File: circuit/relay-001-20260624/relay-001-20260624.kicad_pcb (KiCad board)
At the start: 2 copper layers, 169 x 126.3 mm, 15 parts, among them J1 Conn_01x03_Pin, J10 Conn_01x02_Pin, J11 Conn_01x02_Pin, J12 Conn_01x02_Pin, J13 Conn_01x02_Pin, J14 Conn_01x02_Pin, J15 Conn_01x02_Pin, J2 Conn_02x05_Odd_Even, J3 Conn_02x08_Odd_Even, J4 Conn_02x09_Odd_Even, J5 Conn_01x02_Pin, J6 Conn_01x02_Pin, J7 Conn_01x02_Pin, J8 Conn_01x02_Pin, J9 Conn_01x02_Pin

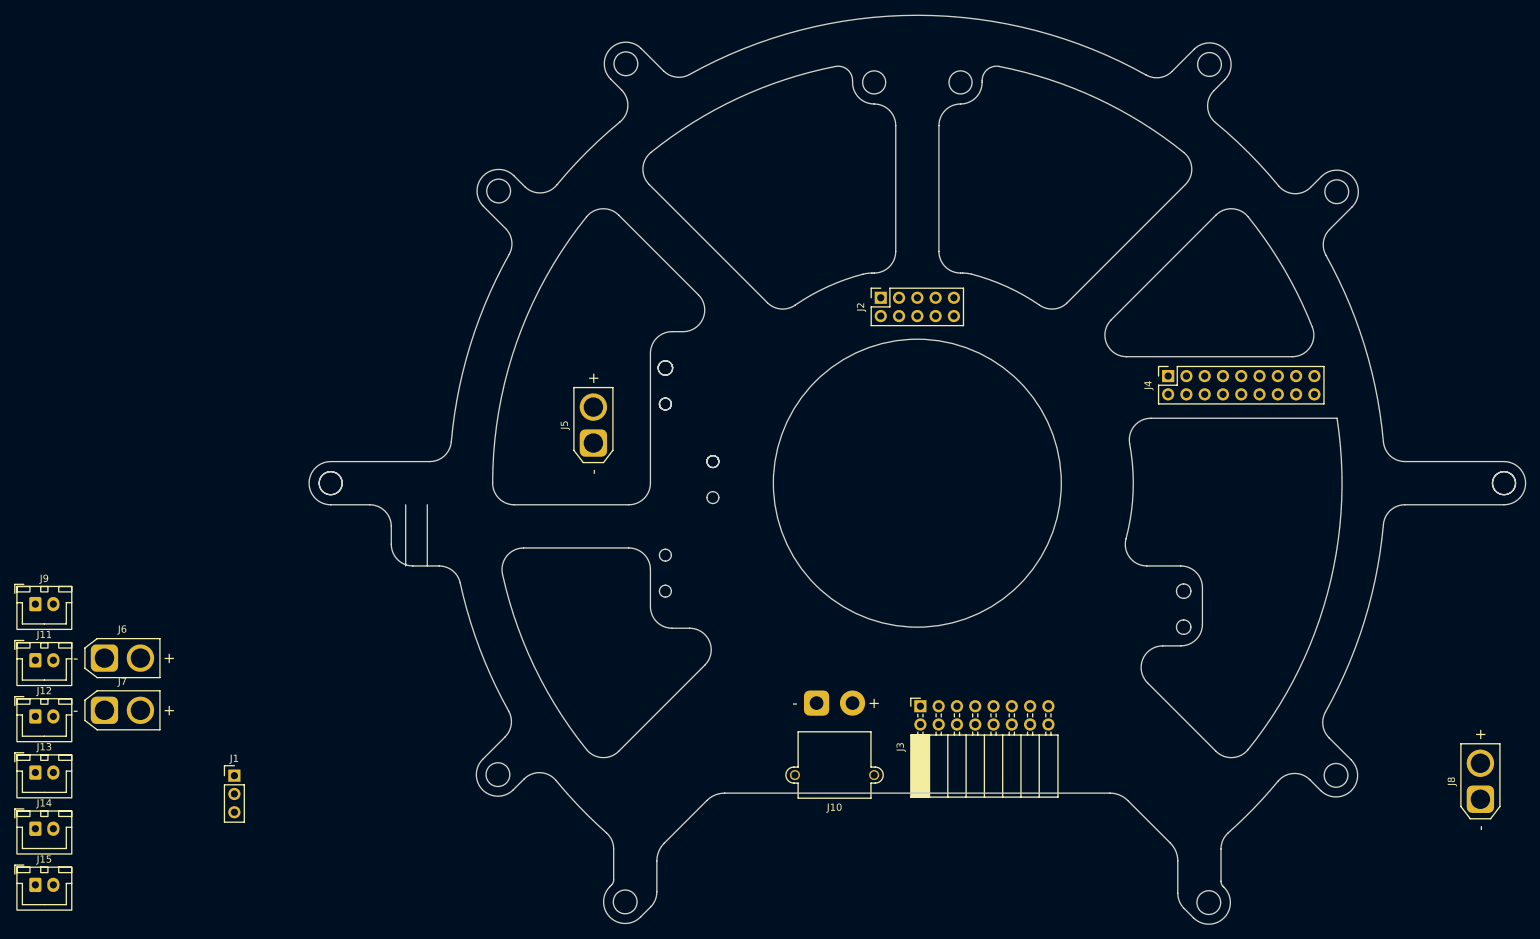
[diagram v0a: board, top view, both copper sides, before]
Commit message: Update 供給基板のボード図を進めた
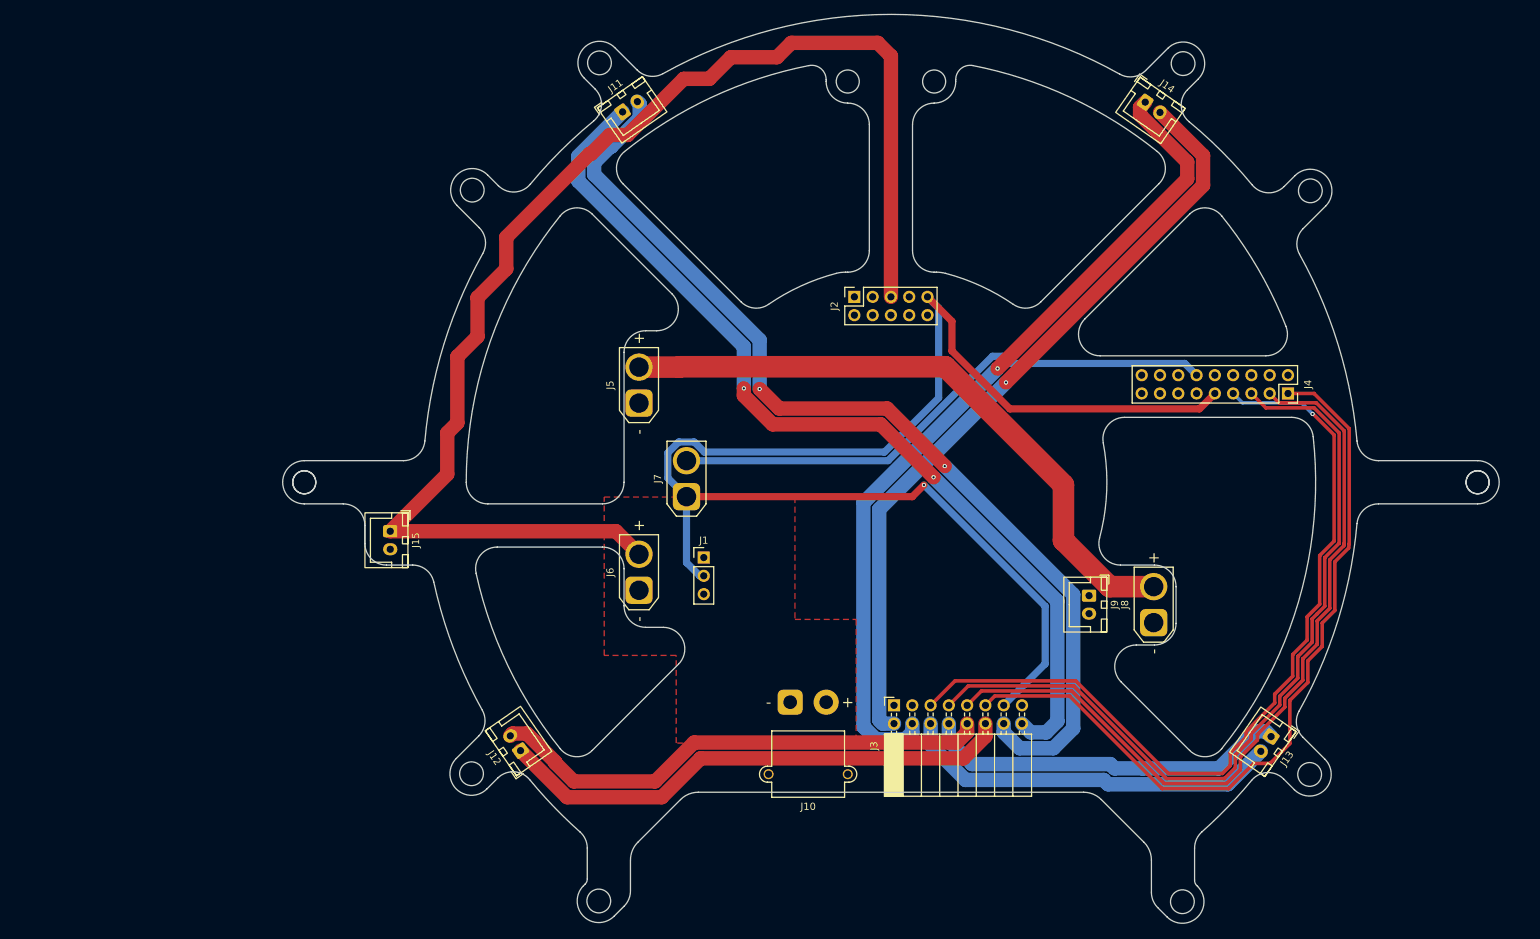
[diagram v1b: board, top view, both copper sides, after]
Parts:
- moved J14 184.3 mm to (185.2, 35.6), turned to -34.8 degrees
- moved J13 171.7 mm to (202.6, 123.8), turned to -124.8 degrees
- moved J9 146.4 mm to (177.4, 104.2), turned to -90 degrees
- moved J11 111.6 mm to (112.6, 37.0), turned to 34.8 degrees
- moved J7 86.1 mm to (121.4, 90.4), turned to 90 degrees
- moved J6 74.9 mm to (114.8, 103.4), turned to 90 degrees
- moved J1 71.9 mm to (123.8, 98.9)
- moved J15 69.6 mm to (80.3, 95.2), turned to -90 degrees
- moved J12 67.6 mm to (98.4, 125.7), turned to 124.8 degrees
- moved J8 51.6 mm to (186.3, 107.9)
- moved J4 16.8 mm to (205.0, 76.1), turned to -90 degrees
- moved J5 8.42 mm to (114.8, 77.4)
- moved J10 3.67 mm to (135.8, 119.0)
- moved J2 3.67 mm to (144.8, 62.7)
- moved J3 3.67 mm to (150.3, 119.4)
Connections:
- J10 pad 1: VCC -> GND
- J10 pad 2: GND -> VCC
- J2 pad 1: GND -> EN_{Boost}
- J2 pad 10: +3.3V -> GND
- J2 pad 2: EN_{Boost} -> GND
- J2 pad 3: EN_{Dribbler-Front} -> Kick_{Chip}
- J2 pad 4: Kick_{Chip} -> EN_{Dribbler-Front}
- J2 pad 5: PH_{Dribbler-Front} -> VCC
- J2 pad 6: VCC -> PH_{Dribbler-Front}
- J2 pad 7: BallCatch_{Front} -> Kick_{Stroke}
- J2 pad 8: Kick_{Stroke} -> BallCatch_{Front}
- J2 pad 9: GND -> +3.3V
- J3 pad 1: Motor_{OUT1-1} -> BallCatch_{Back}
- J3 pad 10: Motor2_{PWM} -> Motor_{OUT2-2}
- J3 pad 11: Motor_{OUT3-2} -> Motor_{EN}
- J3 pad 12: Motor3_{PWM} -> Motor_{OUT2-1}
- J3 pad 13: Motor_{OUT4-1} -> +3.3V
- J3 pad 14: Motor4_{PWM} -> Motor_{OUT1-2}
- J3 pad 15: Motor_{OUT4-2} -> GND
- J3 pad 16: BallCatch_{Back} -> Motor_{OUT1-1}
- J3 pad 2: +3.3V -> Motor_{OUT4-2}
- J3 pad 3: Motor_{OUT1-2} -> Motor4_{PWM}
- J3 pad 4: GND -> Motor_{OUT4-1}
- J3 pad 5: Motor_{OUT2-1} -> Motor3_{PWM}
- J3 pad 6: Motor_{EN} -> Motor_{OUT3-2}
- J3 pad 7: Motor_{OUT2-2} -> Motor2_{PWM}
- J3 pad 8: Motor1_{PWM} -> Motor_{OUT3-1}
- J3 pad 9: Motor_{OUT3-1} -> Motor1_{PWM}
- J5 pad 1: +5V_{Line} -> GND
- J5 pad 2: GND -> +5V_{Line}
- J6 pad 1: VCC -> GND
- J6 pad 2: GND -> VCC
- J7 pad 1: +5V -> +3.3V
- J7 pad 2: +3.3V -> +5V
- J8 pad 1: +5V_{Line} -> GND
- J8 pad 2: GND -> +5V_{Line}
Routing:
- net +3.3V: track 0.00 -> 199.4 mm, vias 0 -> 1
- net VCC: track 0.00 -> 182.2 mm
- net Motor_{OUT1-2}: track 0.00 -> 139.2 mm, vias 0 -> 2
- net Motor_{OUT1-1}: track 0.00 -> 129.6 mm, vias 0 -> 2
- net Motor_{OUT4-1}: track 0.00 -> 117.5 mm, vias 0 -> 1
- net Motor3_{PWM}: track 0.00 -> 117.1 mm, vias 0 -> 1
- net Motor2_{PWM}: track 0.00 -> 113.9 mm
- net Motor1_{PWM}: track 0.00 -> 110.5 mm
- net Motor_{EN}: track 0.00 -> 108.4 mm
- net Motor_{OUT4-2}: track 0.00 -> 107.8 mm, vias 0 -> 1
- net +5V_{Line}: track 0.00 -> 88.7 mm
- net +5V: track 0.00 -> 78.0 mm
- net Motor_{OUT2-1}: track 0.00 -> 72.5 mm
- net Motor_{OUT2-2}: track 0.00 -> 70.5 mm
- net Motor_{OUT3-2}: track 0.00 -> 53.0 mm
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- added copper zone on F.Cu, net VCC
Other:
- outline, holes or cut-outs redrawn
